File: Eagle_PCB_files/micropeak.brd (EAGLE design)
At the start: 18 x 14 mm, 15 parts, among them U1 ATTINY85-20MUR, U2 MS5611-01BA03

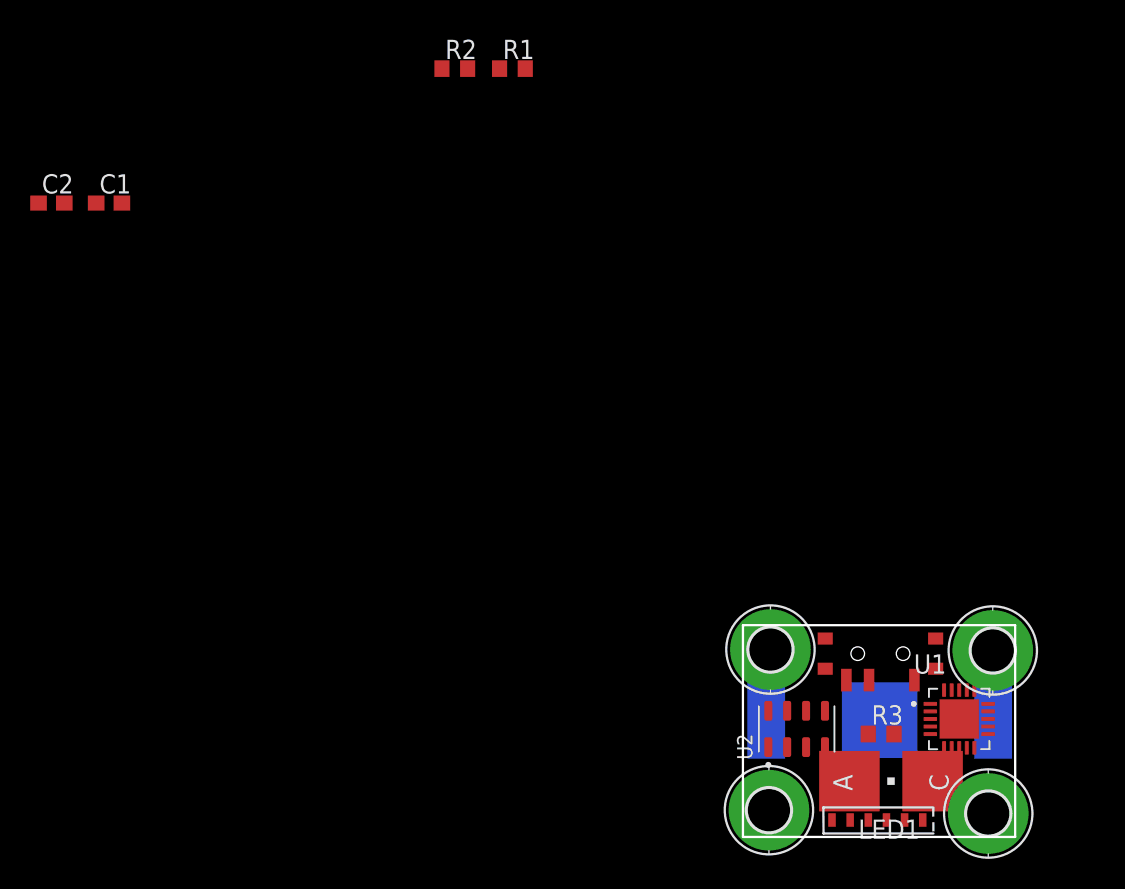
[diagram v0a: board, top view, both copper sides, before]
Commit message: have holes and outline positioned correctly - floorplanning done pretty much
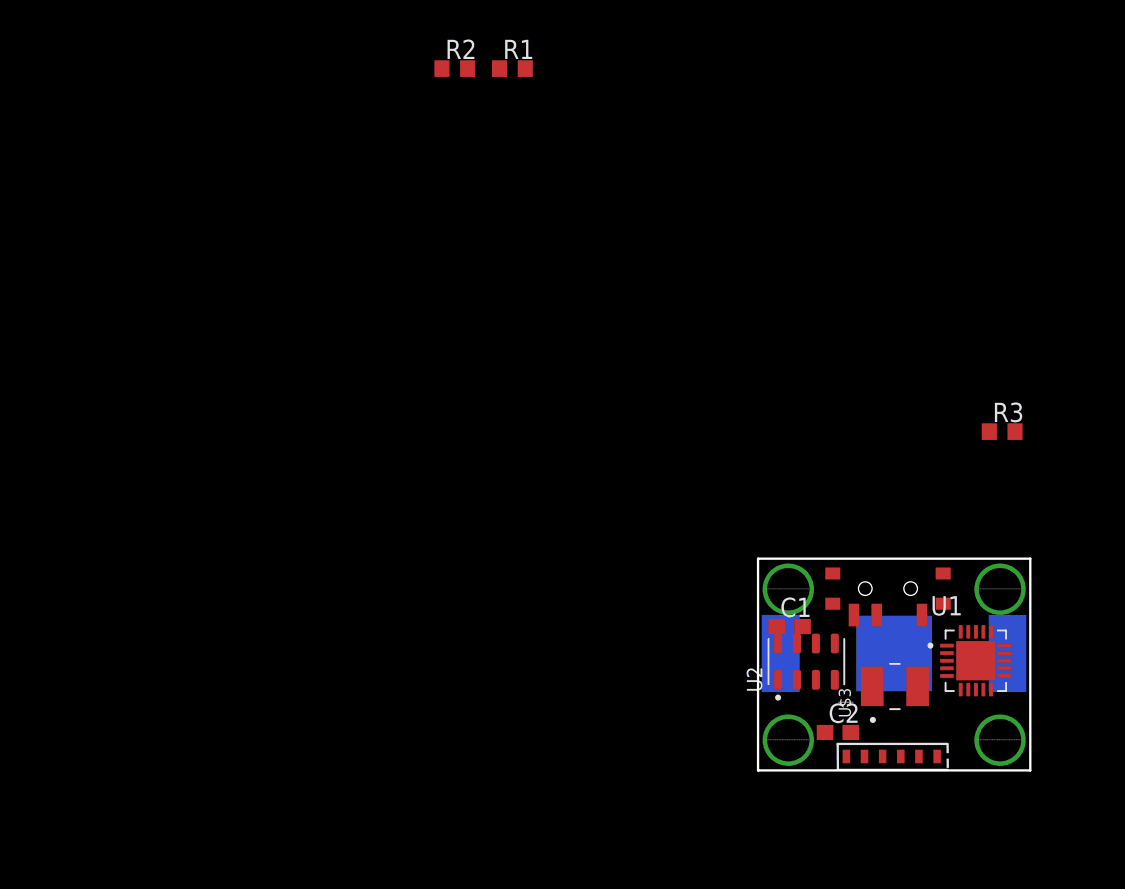
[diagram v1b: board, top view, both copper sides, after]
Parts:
- removed H1, H2, H3, H4: MOUNT-PAD-ROUND2.8, holes:2,8-PAD
- removed LED1: (no value), led:P-LCC-2
- added U$3: LED, LED_LYT68B-T2V1-26-Z:LED_LYT68B-T2V1-26-Z
- added U$4, U$5, U$6, U$7: (no value), LED_LYT68B-T2V1-26-Z:2,8-PAD
- moved C2 62.7 mm to (6.28, 6.91)
- moved C1 53.0 mm to (3.09, 13.9)
- moved R3 21.5 mm to (17.1, 26.8)
- moved BT1 4.50 mm to (9.99, 12.1)
- moved U2 4.50 mm to (4.20, 11.6)
- moved U$1 4.33 mm to (9.59, 16.4)
- moved U$2 4.31 mm to (12.8, 5.32)
- moved U1 4.00 mm to (15.4, 11.7)
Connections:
- net +3V3: now also U$4.B2,8, U$5.B2,8, U$6.B2,8, U$7.B2,8; no longer H1.B2,8, H2.B2,8, H3.B2,8, H4.B2,8
- net GND: now also U$3.C; no longer LED1.C
- net N$4: now also U$3.A; no longer LED1.A

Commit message: routing done
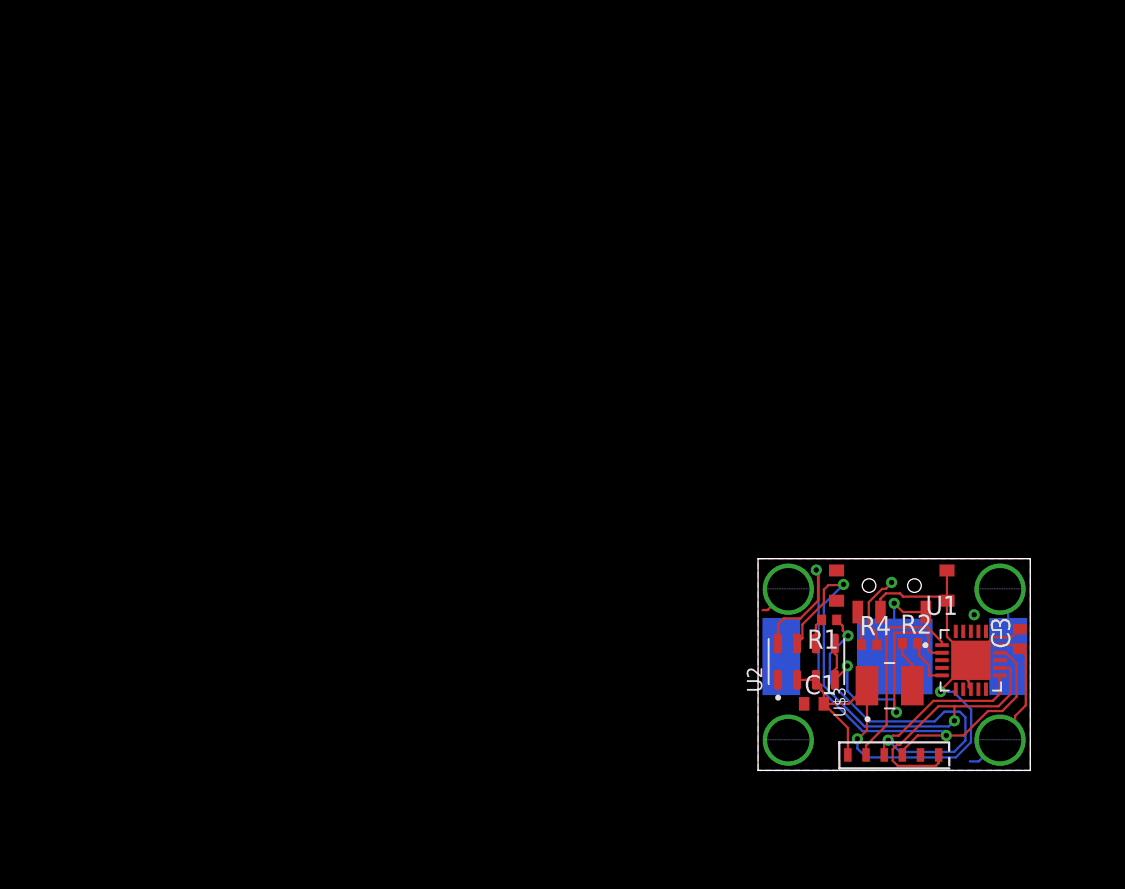
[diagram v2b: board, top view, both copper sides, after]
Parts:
- removed C2: (no value), rcl:C0603
- removed R3: (no value), rcl:R0603
- added C3: (no value), rcl:C0402
- added R4: (no value), rcl:R0402
- C1: device rcl:C0603 -> rcl:C0402
- R1, R2: device rcl:R0603 -> rcl:R0402
- moved R2 48.5 mm to (11.1, 12.8)
- moved R1 42.0 mm to (5.70, 14.3), turned to 180 degrees
- moved C1 5.36 mm to (4.70, 8.80)
- moved U$3 0.35 mm to (9.70, 10.0)
- moved U1 0.33 mm to (15.1, 11.7)
- moved U$1 0.32 mm to (9.84, 16.6)
- moved BT1 0.21 mm to (10.0, 11.9)
- moved U$2 0.14 mm to (12.9, 5.42)
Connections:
- new net N$11: U$1.P$6
- new net N$12: U$1.P$7
- net +3V3: now also C3.1, R4.2; no longer C2.1, R2.2
- net GND: now also C3.2; no longer C2.2, U$1.P$6, U$1.P$7
- net MOSI: now also R1.1; no longer R3.1
- net N$2: now also R4.1; no longer R2.1
- net N$3: now also R2.2; no longer R1.1
- net N$4: now also R2.1; no longer R1.2
- net N$5: now also R1.2; no longer R3.2
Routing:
- net GND: track 0.00 -> 50.3 mm, vias 0 -> 2
- net MISO: track 0.00 -> 40.1 mm, vias 0 -> 2
- net SCK: track 0.00 -> 37.3 mm, vias 0 -> 2
- net MOSI: track 0.00 -> 33.6 mm, vias 0 -> 2
- net +3V3: track 0.00 -> 23.2 mm, vias 0 -> 1
- net CS_BARO: track 0.00 -> 19.2 mm, vias 0 -> 2
- net !RESET!: track 0.00 -> 13.1 mm
- net N$1: track 0.00 -> 5.87 mm, vias 0 -> 1
- net N$3: track 0.00 -> 3.28 mm
- net N$4: track 0.00 -> 3.07 mm
- net N$2: track 0.00 -> 2.28 mm
- net N$5: track 0.00 -> 1.72 mm
- added copper zone on layer 1, net +3V3
- added copper zone on layer 16, net +3V3
